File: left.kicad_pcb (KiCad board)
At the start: 2 copper layers, 152.4 x 109.7 mm, 67 parts, among them U1 74VHC4051AFT, U2 GS8051-TR, U3 ATMEGA32U4, U4 PJ-327A, Y1 Crystal

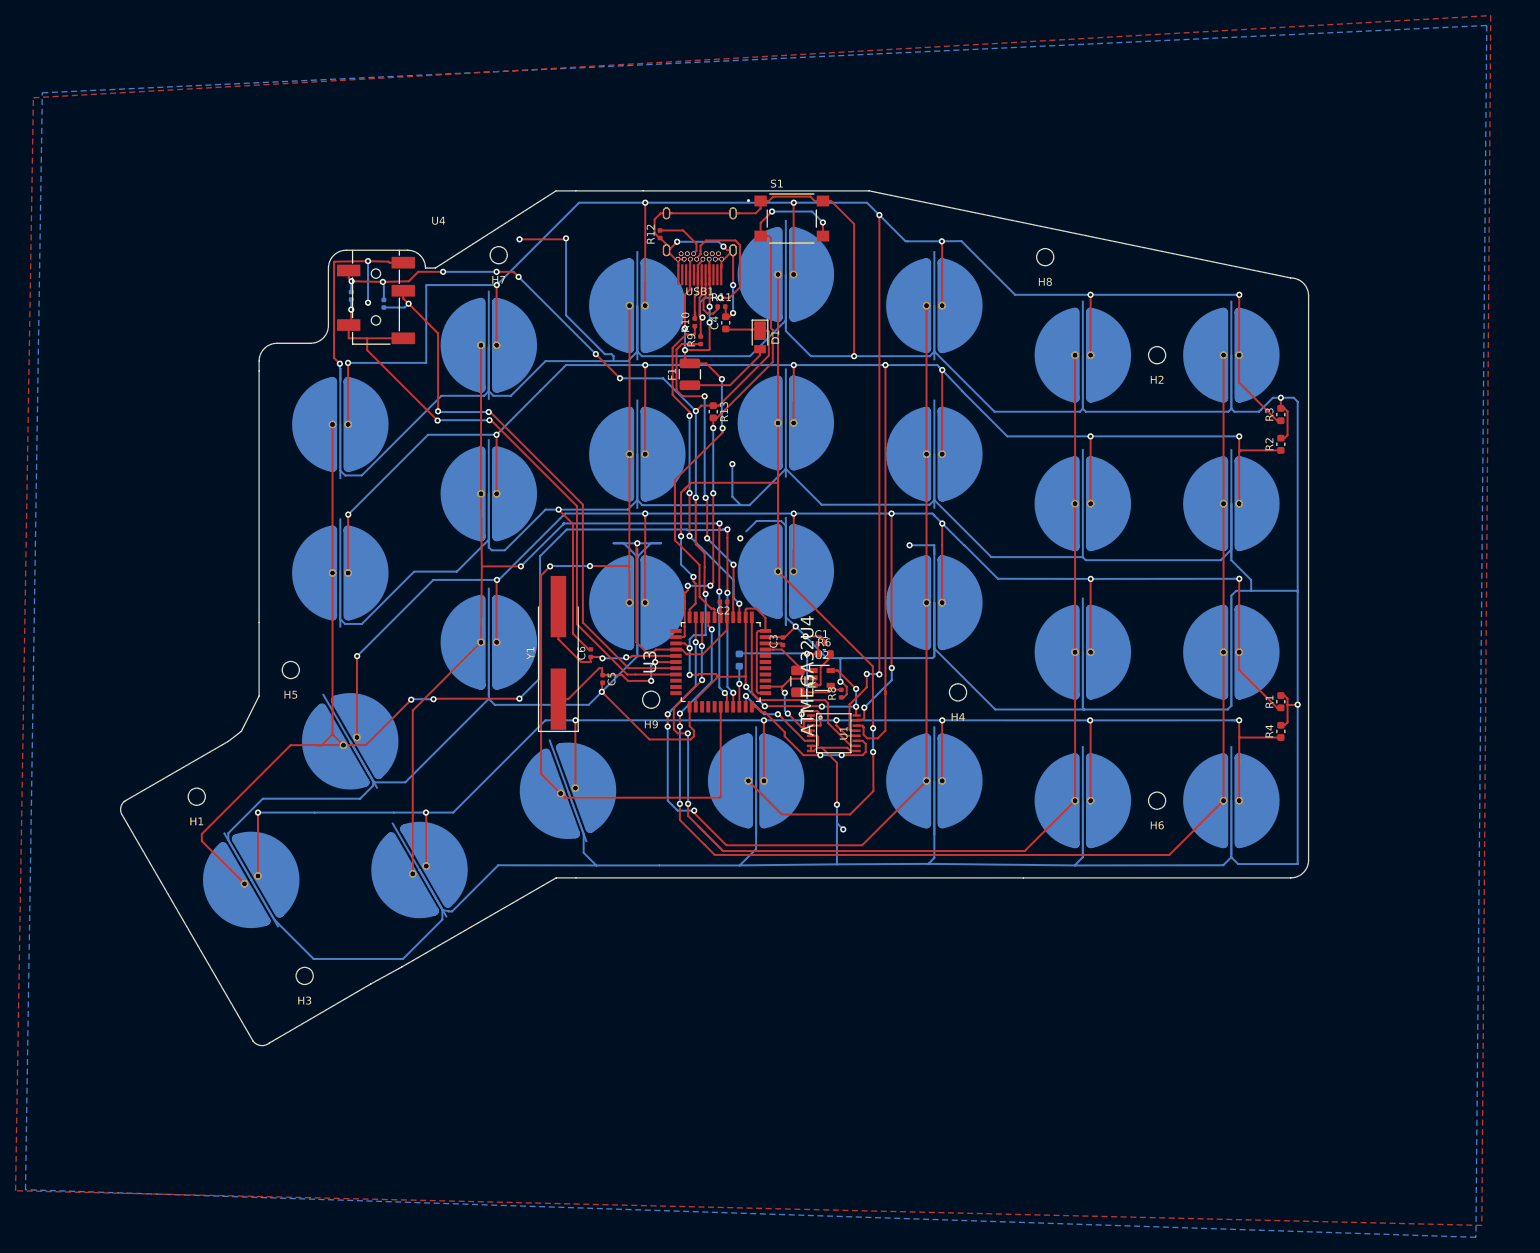
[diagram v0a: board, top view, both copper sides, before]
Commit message: fix jack
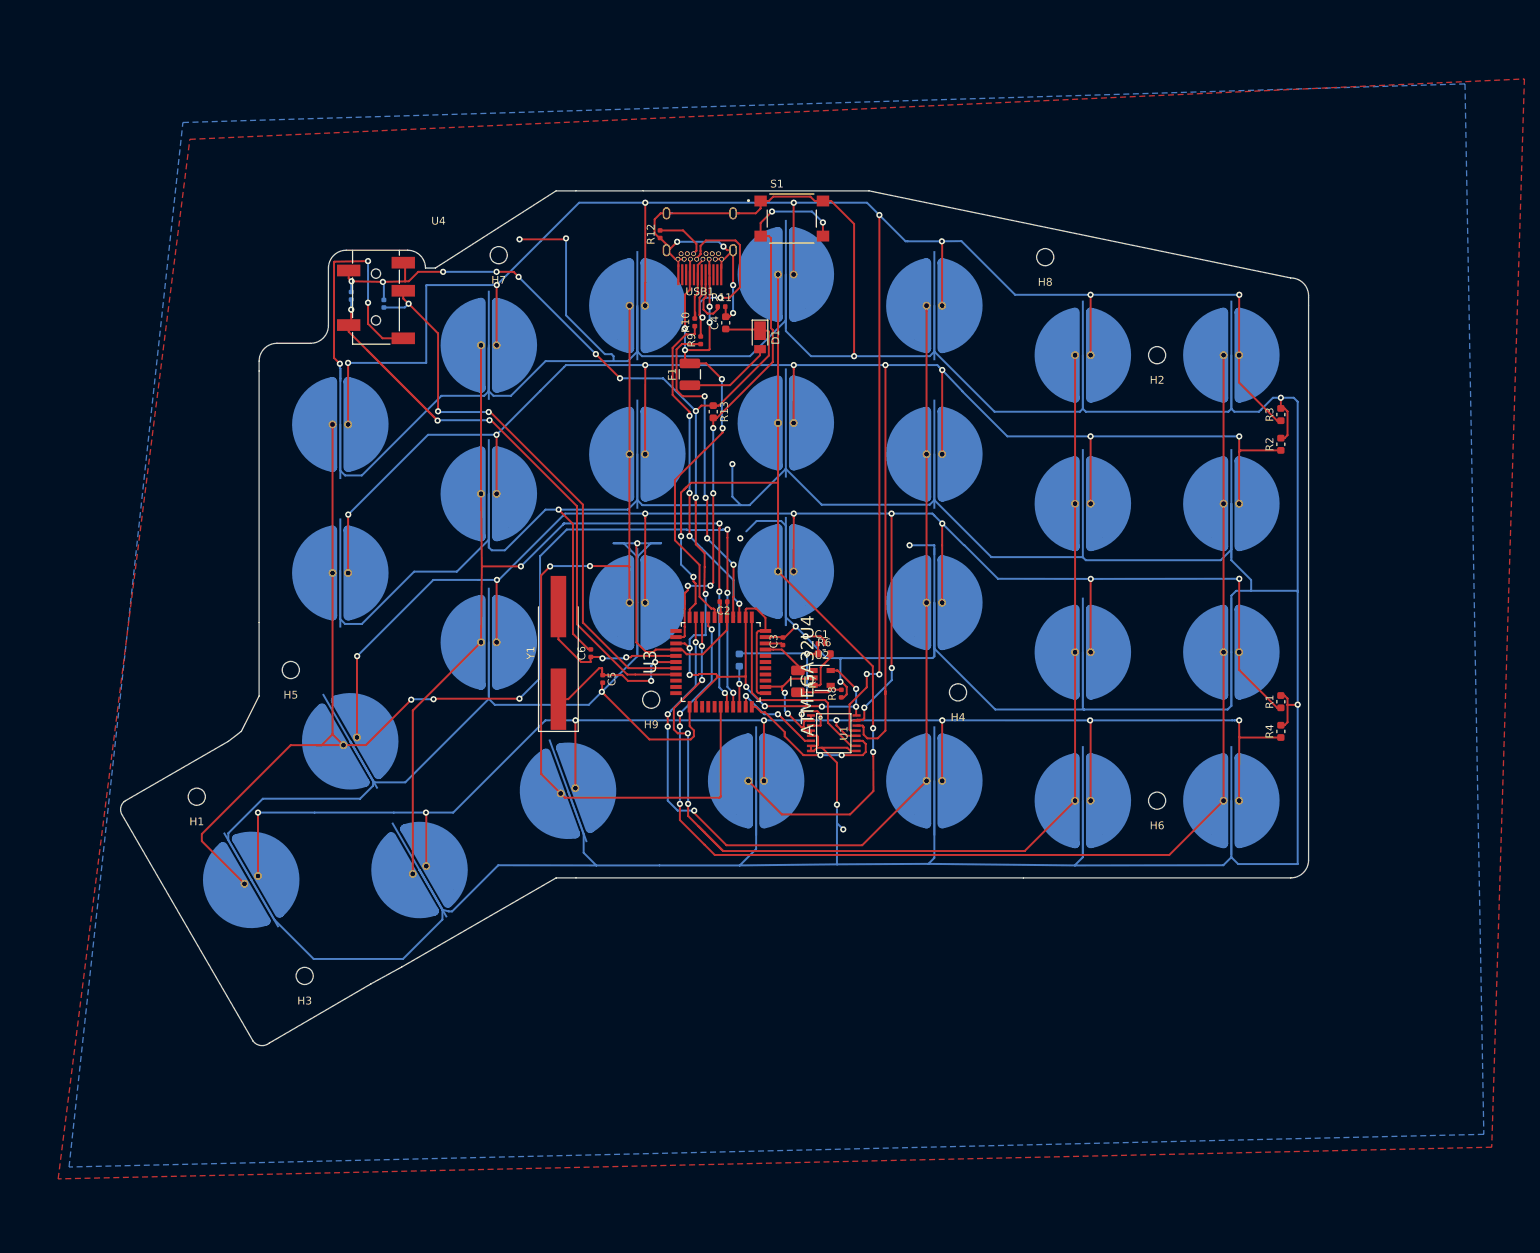
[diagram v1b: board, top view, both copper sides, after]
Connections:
- U4 pad 4: GND -> VCC
- U4 pad 6: sda -> GND
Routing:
- net sda: track 78.7 -> 86.1 mm
- net GND: track 1178.2 -> 1181.6 mm
- net VCC: track 177.9 -> 180.4 mm
